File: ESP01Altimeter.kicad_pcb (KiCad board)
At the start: 2 copper layers, 47 x 17.8 mm, 9 parts, among them SW1 Reset, SW2 Select

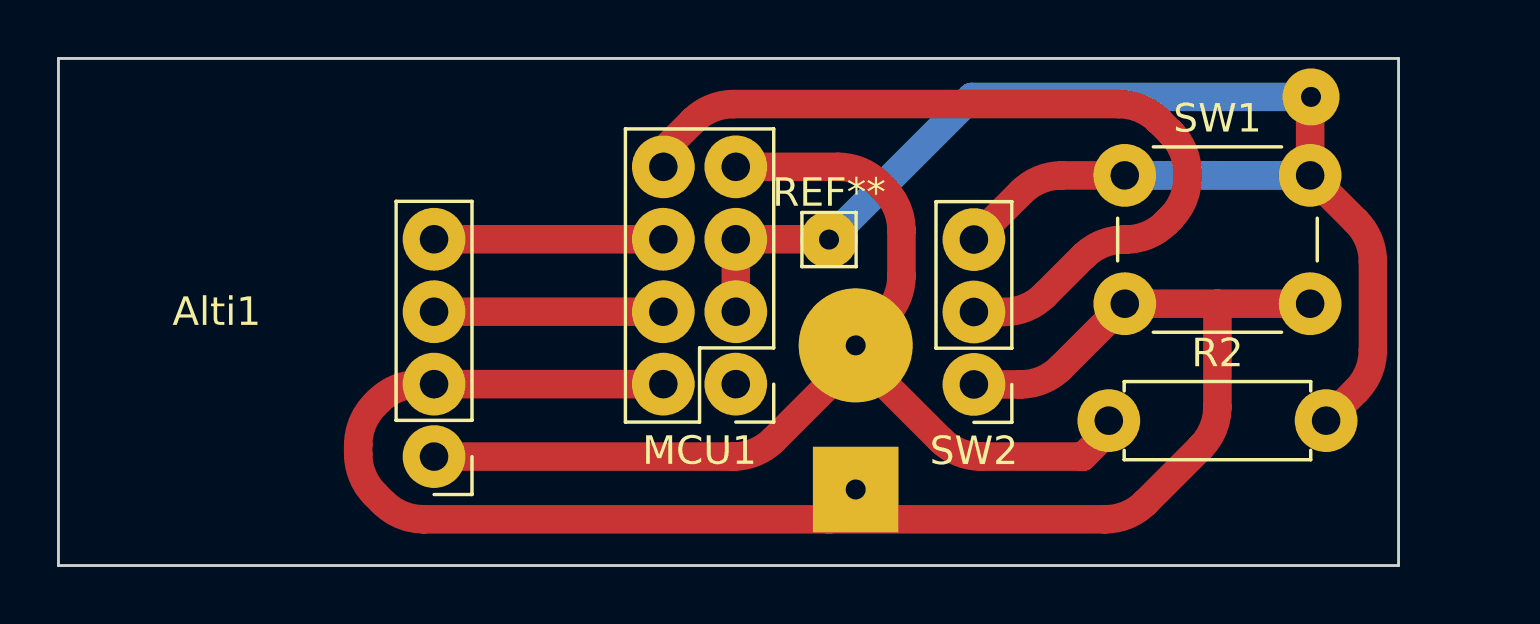
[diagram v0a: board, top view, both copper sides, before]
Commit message: V0.2
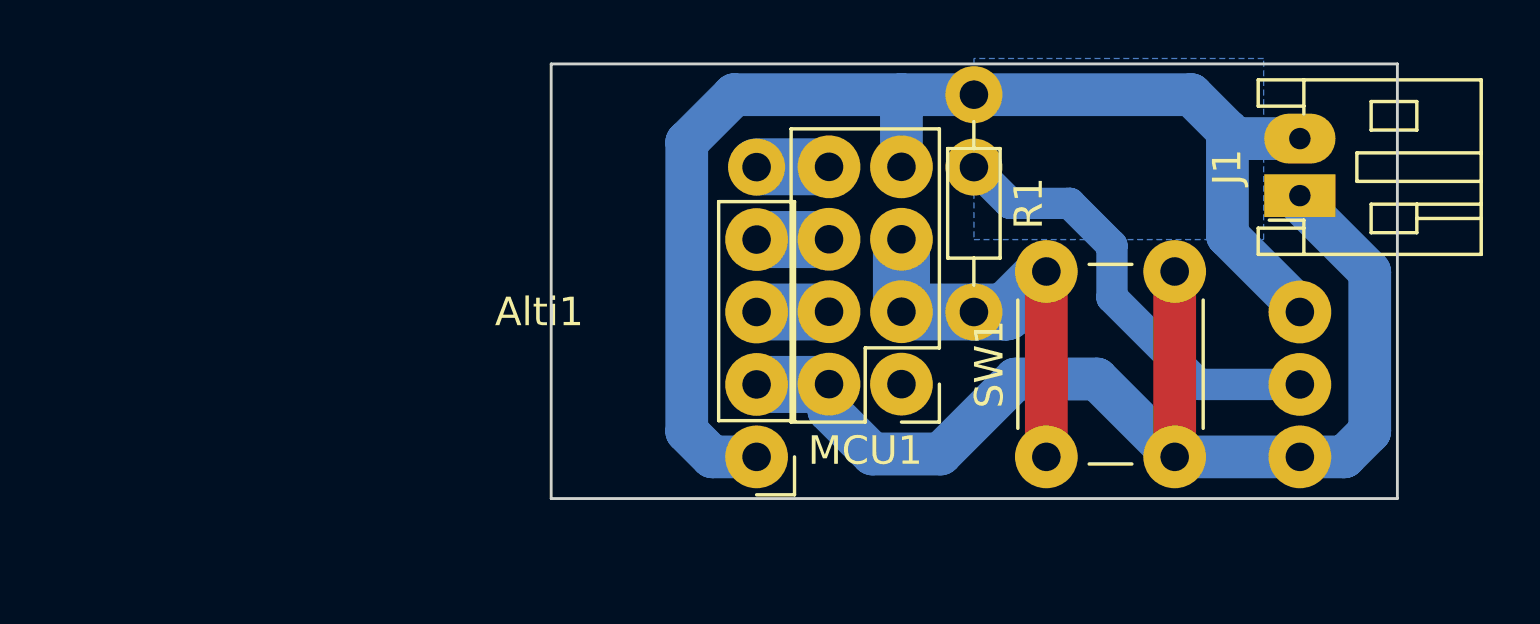
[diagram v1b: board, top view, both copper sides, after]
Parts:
- removed ? (x3): , 
- removed REF**: TestPoint_THTPad_1.5x1.5mm_Drill0.7mm, TestPoint:TestPoint_THTPad_1.5x1.5mm_Drill0.7mm
- added J1: Conn_01x02_Pin, Connector_JST:JST_PH_S2B-PH-K_1x02_P2.00mm_Horizontal, F.Cu at (168.9, 105.1)
- added R2: 10K, Resistor_THT:R_Axial_DIN0204_L3.6mm_D1.6mm_P7.62mm_Horizontal, B.Cu at (149.9, 104.1)
- R1: renamed from R2; footprint Resistor_THT:R_Axial_DIN0207_L6.3mm_D2.5mm_P7.62mm_Horizontal -> Resistor_THT:R_Axial_DIN0204_L3.6mm_D1.6mm_P7.62mm_Horizontal
- SW2: moved to B.Cu
- moved R1 12.4 mm to (157.5, 101.6), turned to -90 degrees
- moved SW2 11.4 mm to (168.9, 111.8)
- moved Alti1 11.3 mm to (149.9, 114.3)
- moved SW1 10.2 mm to (160.0, 114.3), turned to 90 degrees
- moved MCU1 5.81 mm to (154.9, 111.8)
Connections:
- SW2 pad 1: GND -> +3V3
- SW2 pad 2: Net-(MCU1-GPIO3) -> Net-(SW2-B)
- SW2 pad 3: Net-(MCU1-CH_PD) -> GND
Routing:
- net Net-(MCU1-CH_PD): track 50.2 -> 14.7 mm
- net Net-(MCU1-GPIO3): track 30.5 -> 2.54 mm
- net GND: track 63.3 -> 41.2 mm
- net Net-(SW2-B): track 0.00 -> 15.7 mm
- net +3V3: track 40.5 -> 46.3 mm
- net Net-(Alti1-SDA): track 8.16 -> 2.54 mm
- net Net-(Alti1-SCL): track 8.04 -> 2.54 mm
- added copper zone on B.Cu, net +3V3
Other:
- board size 47 x 17.8 mm -> 29.7 x 15.2 mm
- board text added: "DR&LM"
- board text added: "Titania"
